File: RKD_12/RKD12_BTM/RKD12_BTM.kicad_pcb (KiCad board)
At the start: 2 copper layers, 98.8 x 97.7 mm, 25 parts

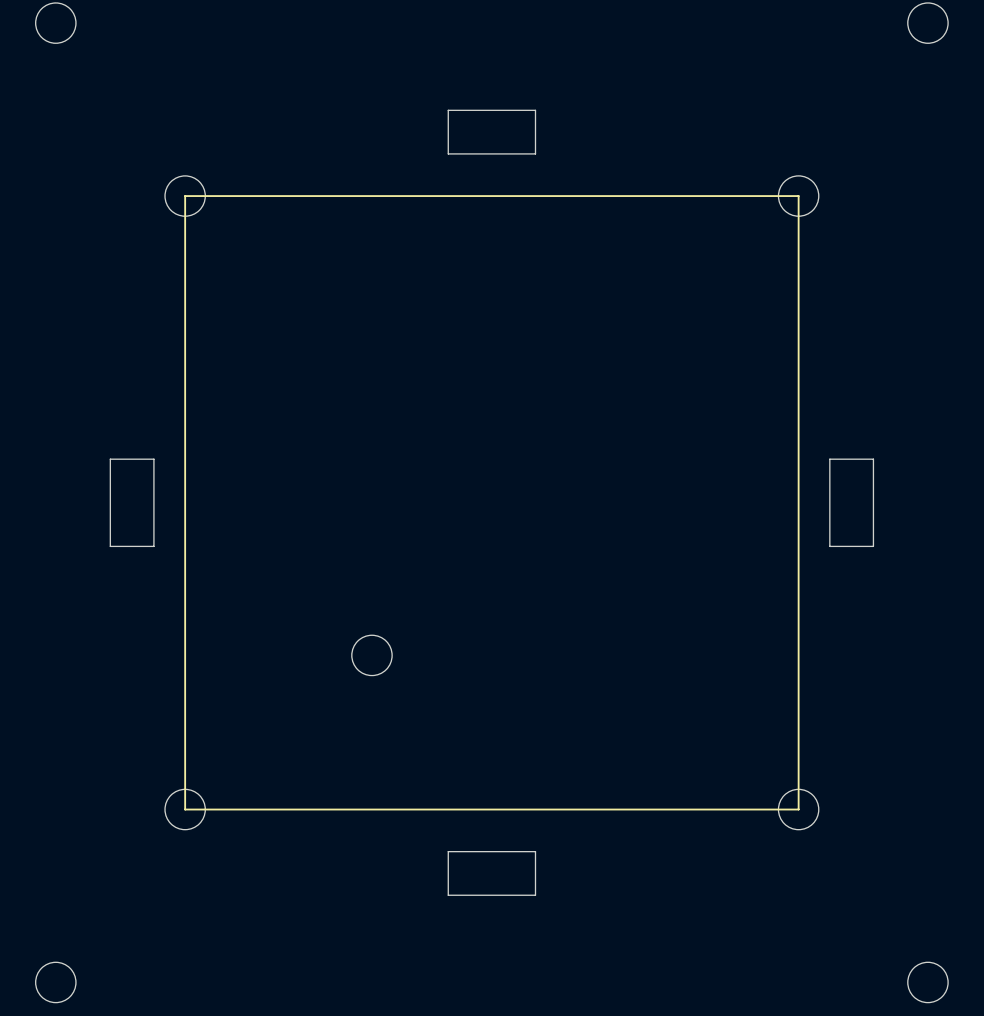
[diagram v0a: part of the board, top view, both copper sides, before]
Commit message: Combine
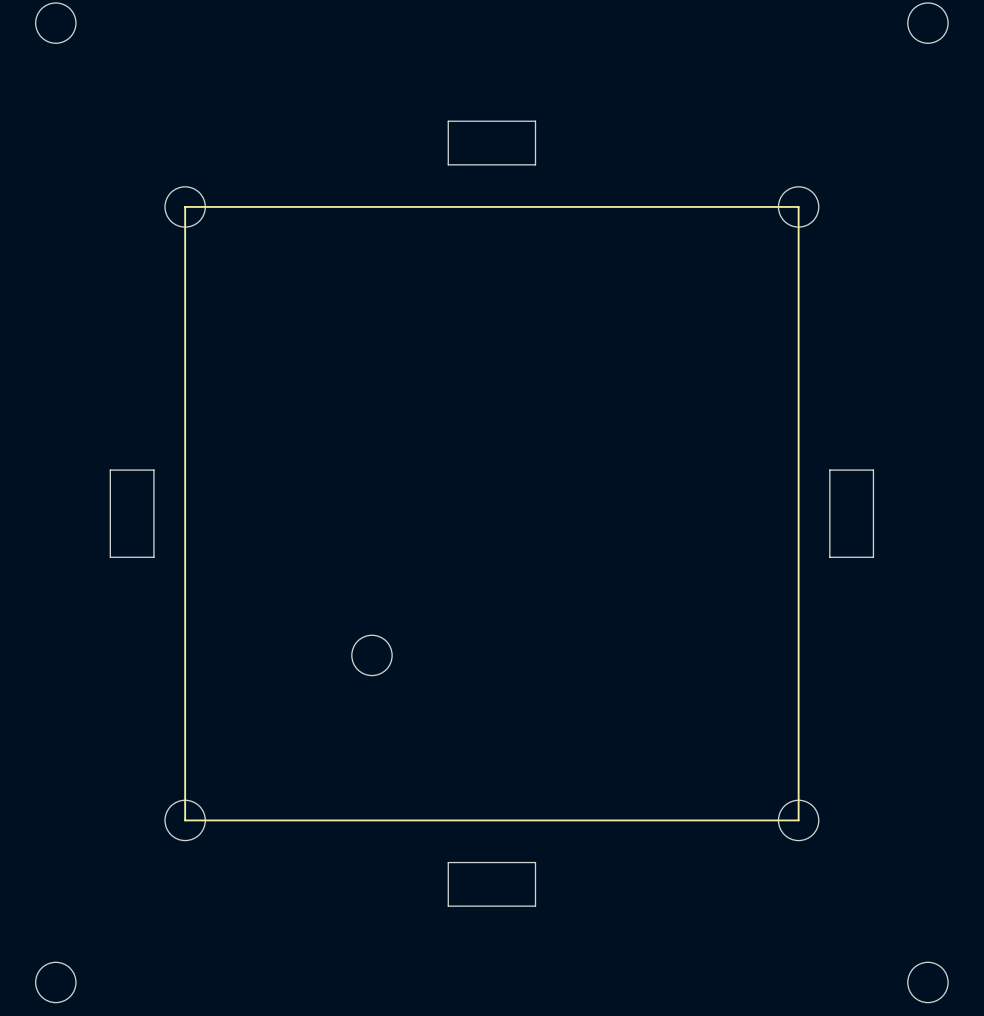
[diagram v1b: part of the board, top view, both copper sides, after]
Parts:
- moved Picot** 0.60 mm to (128.0, 75.6)
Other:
- outline, holes or cut-outs redrawn
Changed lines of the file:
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@@
 	(footprint "Rikkodo_FootPrint:rkd_picot5400_BTM"
 		(layer "F.Cu")
-		(at 127.992295 75.009438)
+		(at 127.992295 75.604713)
 		(property "Reference" "Picot**"
 			(at 0 -0.5 0)
@@
 	)
 	(gr_circle
-		(center 127.992329 75.009476)
-		(end 130.373579 75.009476)
+		(center 127.992329 75.604751)
+		(end 130.373579 75.604751)
 		(stroke
 			(width 0.1)
@@
 	)
 	(gr_line
-		(start 127.992329 55.959375)
-		(end 127.992329 94.059375)
+		(start 127.992329 56.55465)
+		(end 127.992329 94.65465)
 		(stroke
 			(width 0.1)
@@
 	)
 	(gr_line
-		(start 146.446875 75.009375)
-		(end 109.5375 75.009476)
+		(start 146.446875 75.60465)
+		(end 109.5375 75.604751)
 		(stroke
 			(width 0.1)
@@
 	)
 	(gr_rect
-		(start 125.611078 94.059375)
-		(end 130.37358 96.440625)
+		(start 125.611078 94.65465)
+		(end 130.37358 97.0359)
 		(stroke
 			(width 0.05)
@@
 	)
 	(gr_rect
-		(start 146.446875 72.628124)
-		(end 148.828125 77.390626)
+		(start 146.446875 73.223399)
+		(end 148.828125 77.985901)
 		(stroke
 			(width 0.05)
@@
 	)
 	(gr_rect
-		(start 107.156342 72.628187)
-		(end 109.537592 77.390689)
+		(start 107.156342 73.223462)
+		(end 109.537592 77.985964)
 		(stroke
 			(width 0.05)
@@
 	)
 	(gr_rect
-		(start 125.611078 53.578125)
-		(end 130.37358 55.959375)
+		(start 125.611078 54.1734)
+		(end 130.37358 56.55465)
 		(stroke
 			(width 0.05)
